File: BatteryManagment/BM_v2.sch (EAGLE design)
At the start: 163 parts, among them U1 ATMEGA328P-AU

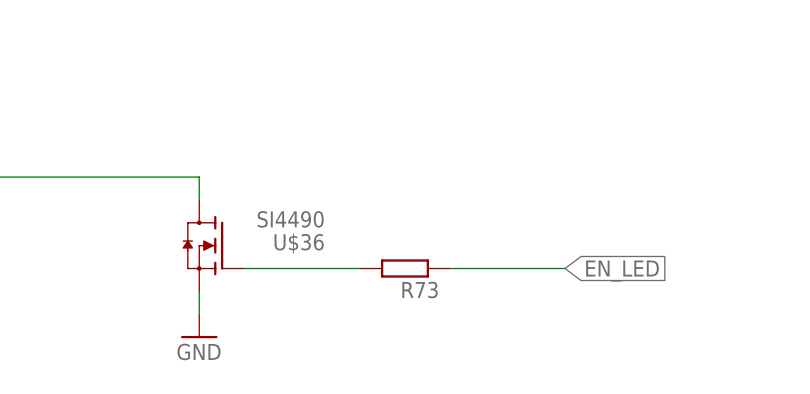
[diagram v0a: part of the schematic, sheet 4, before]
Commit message: backup
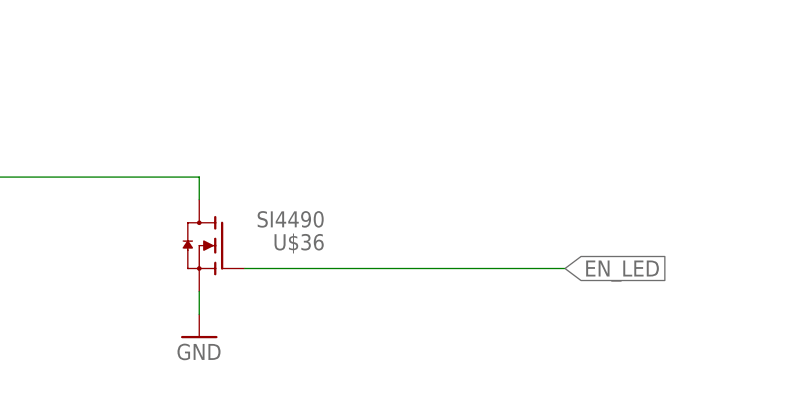
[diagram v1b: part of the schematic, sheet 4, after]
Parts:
- removed R73: (no value), rcl:R-EU_R0603
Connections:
- removed net N$57: R73.2, U$36.G
- net EN_LED: now also U$36.G; no longer R73.1
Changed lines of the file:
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@@
 <part name="U$36" library="BM_pre" deviceset="SI4490" device=""/>
 <part name="GND29" library="supply1" deviceset="GND" device=""/>
-<part name="R73" library="rcl" deviceset="R-EU_" device="R0603"/>
 <part name="R74" library="rcl" deviceset="R-EU_" device="R0603" value="0"/>
 <part name="R75" library="rcl" deviceset="R-EU_" device="R0603" value="0"/>
@@
 <instance part="U$36" gate="G$1" x="139.7" y="63.5" rot="MR0"/>
 <instance part="GND29" gate="1" x="137.16" y="53.34"/>
-<instance part="R73" gate="G$1" x="160.02" y="60.96" rot="R180"/>
 <instance part="15V" gate="1" x="68.58" y="99.06"/>
 </instances>
@@
 </segment>
 </net>
-<net name="N$57" class="0">
-<segment>
+<net name="EN_LED" class="0">
+<segment>
+<label x="177.8" y="60.96" size="1.778" layer="95" xref="yes"/>
 <pinref part="U$36" gate="G$1" pin="G"/>
-<pinref part="R73" gate="G$1" pin="2"/>
-<wire x1="142.24" y1="60.96" x2="154.94" y2="60.96" width="0.1524" layer="91"/>
-</segment>
-</net>
-<net name="EN_LED" class="0">
-<segment>
-<pinref part="R73" gate="G$1" pin="1"/>
-<wire x1="165.1" y1="60.96" x2="177.8" y2="60.96" width="0.1524" layer="91"/>
-<label x="177.8" y="60.96" size="1.778" layer="95" xref="yes"/>
-</segment>
-</net>
+<wire x1="142.24" y1="60.96" x2="177.8" y2="60.96" width="0.1524" layer="91"/>
+</segment>
+</net>
